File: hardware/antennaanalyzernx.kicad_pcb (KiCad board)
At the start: 2 copper layers, 83.9 x 99 mm, 140 parts, among them J1 Power Connection, J2 SPI Header, J3 Serial Header, J4 GPIO, J5 Conn_Coaxial, J6 TFT Connection, J7 Touch Connection, J8 SD Connection, SW1 Reset, U1 SA612, U10 TLV1117-33, U11 TLV1117-50, U12 ATmega1284P-AU, U2 LM358, U3 Si5351A, U4 SA612, U5 LM358, U6 74HC86, U7 74HC74, U8 LM358, U9 LM324, Y1 27MHz, Y2 16MHz

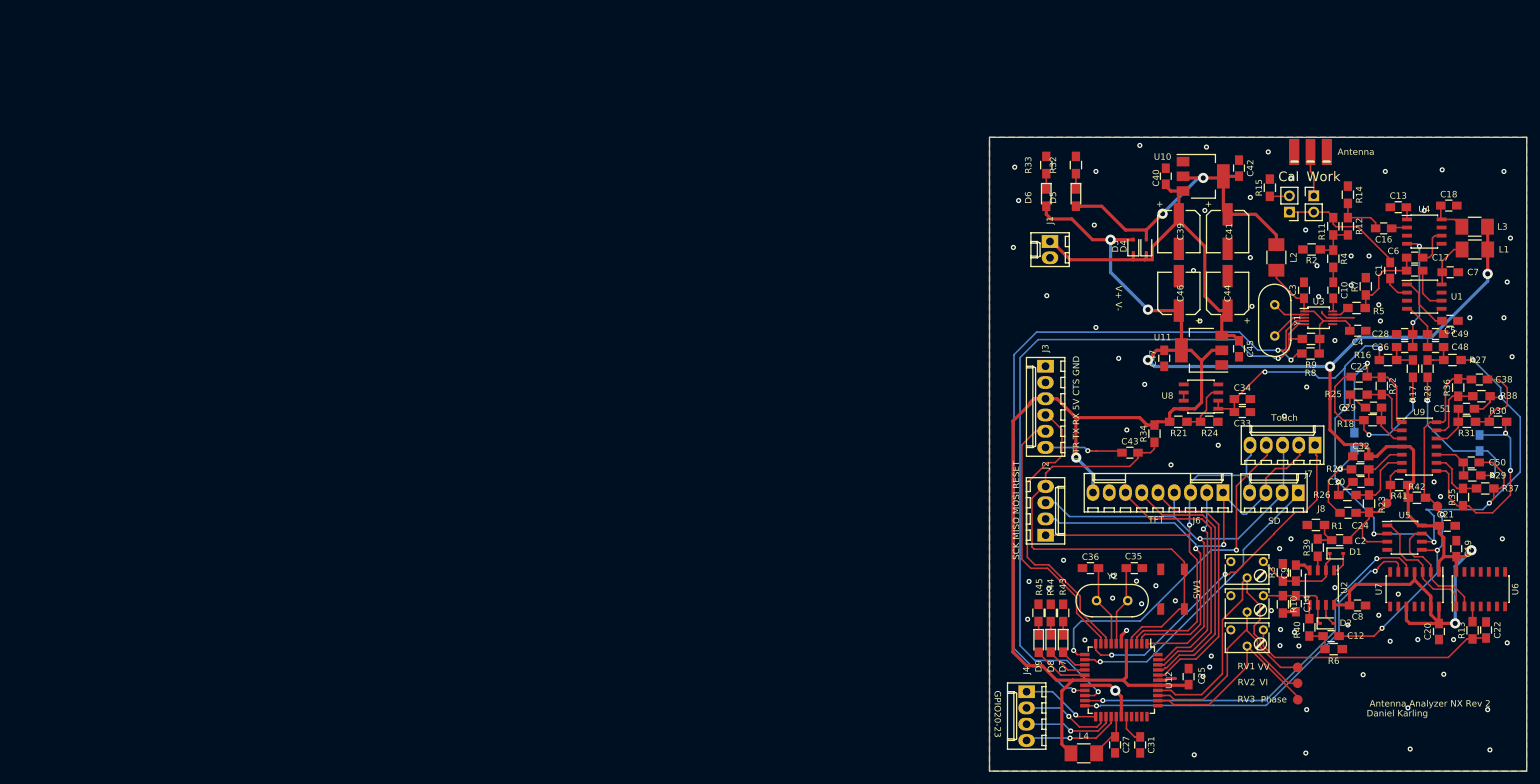
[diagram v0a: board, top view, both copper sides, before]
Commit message: stm32 version
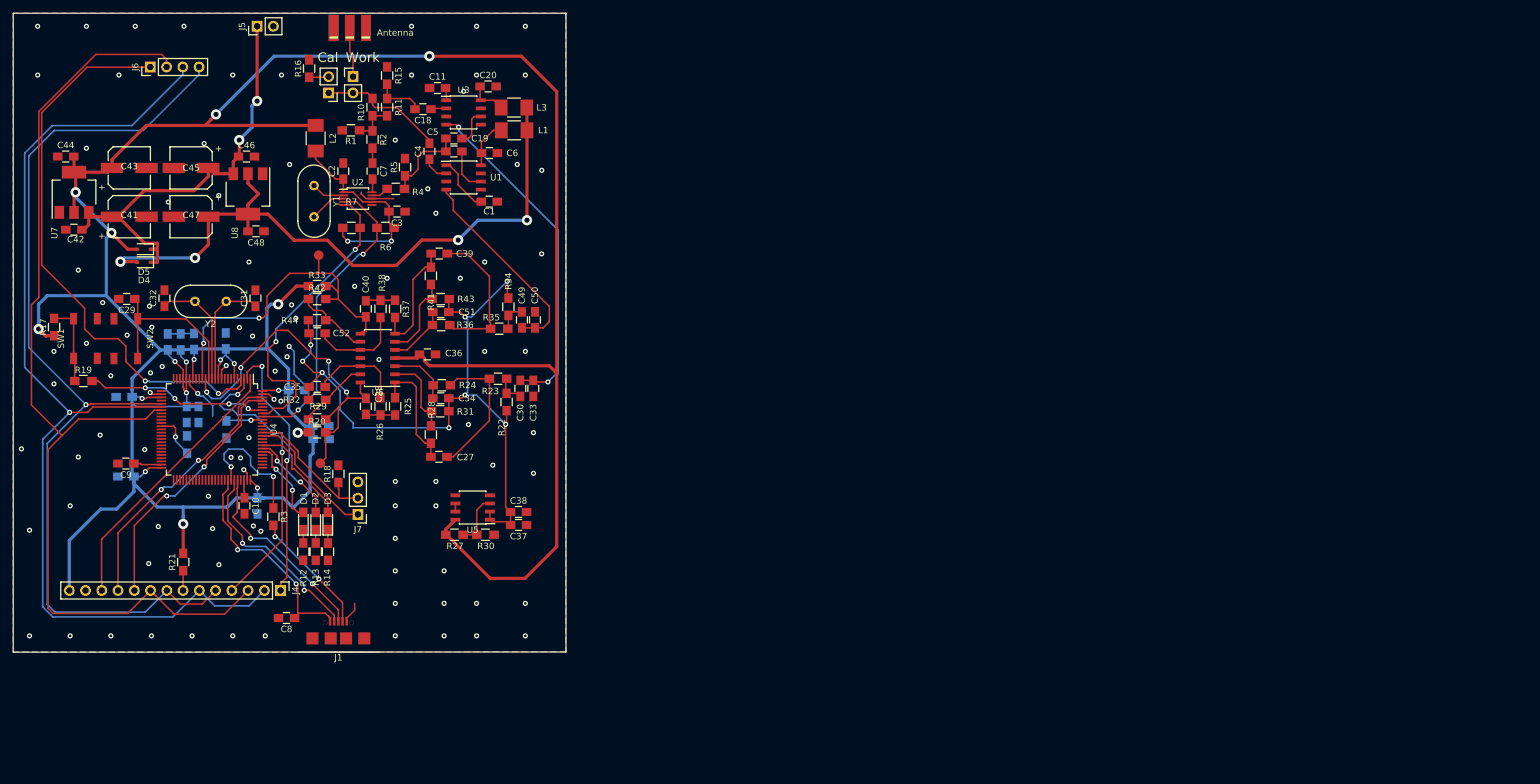
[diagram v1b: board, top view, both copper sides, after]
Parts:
- removed the C19 at (246.8, 103.6)
- removed the C2 at (228.6, 102.3)
- removed the C20 at (244.1, 116.6)
- removed the C27 at (193.5, 134.3)
- removed the C35 at (196.5, 106.7)
- removed the C36 at (189.6, 106.7)
- removed the C43 at (195.8, 88.6)
- removed the D1 at (228.1, 104.4)
- removed the D2 at (226.6, 115.3)
- removed the D5 at (187.4, 48.8)
- removed D6: 5V PWR, LEDs:LED_0805_HandSoldering
- removed the J2 at (182.6, 101.5)
- removed J3: Serial Header, Connectors_Molex:Molex_KK-6410-06_06x2.54mm_Straight
- removed J8: SD Connection, Connectors_Molex:Molex_KK-6410-04_04x2.54mm_Straight
- removed L4: 1u, Inductors_SMD:L_1210_HandSoldering
- removed the R1 at (224.9, 99.9)
- removed the R10 at (219.7, 112.3)
- removed the R13 at (249.3, 116.4)
- removed the R32 at (187.4, 43.7)
- removed the R33 at (182.7, 43.7)
- removed the R34 at (199.6, 85.7)
- removed R39, R40: 10k, Resistors_SMD:R_0805_HandSoldering
- removed the R6 at (227.6, 119.3)
- removed RV1, RV2, RV3: 100k, Potentiometers:Potentiometer_Trimmer_Bourns_3266W
- removed the TP1 at (222.0, 122.2)
- removed the TP2 at (222.0, 124.7)
- removed TP3: TestPoint, Measurement_Points:Measurement_Point_Round-SMD-Pad_Small
- removed U12: ATmega1284P-AU, Housings_QFP:TQFP-44_10x10mm_Pitch0.8mm
- removed the U2 at (225.8, 109.7)
- removed the U7 at (240.3, 110.0)
- removed the U8 at (206.9, 79.9)
- removed U9: LM324, Housings_SOIC:SOIC-14_3.9x8.7mm_Pitch1.27mm
- added C10: 2.2u, Capacitors_SMD:C_0805_HandSoldering, F.Cu at (57.5, 96.9)
- added C13: 100n, Capacitors_SMD:C_0805_HandSoldering, B.Cu at (65.6, 78.9)
- added C15: 100n, Capacitors_SMD:C_0805_HandSoldering, B.Cu at (54.5, 71.2)
- added C16: 100n, Capacitors_SMD:C_0805_HandSoldering, B.Cu at (47.5, 71.3)
- added C17: 100n, Capacitors_SMD:C_0805_HandSoldering, B.Cu at (38.9, 92.4)
- added C23: 4.7u, Capacitors_SMD:C_0805_HandSoldering, B.Cu at (69.4, 86.5)
- added C24: 4.7u, Capacitors_SMD:C_0805_HandSoldering, B.Cu at (69.4, 84.5)
- added C26: 100n, Capacitors_SMD:C_0805_HandSoldering, B.Cu at (38.6, 79.9)
- added C29: 100n, Capacitors_SMD:C_0805_HandSoldering, F.Cu at (39.1, 64.6)
- added C32: 20p, Capacitors_SMD:C_0805_HandSoldering, F.Cu at (45.0, 64.5)
- added J5: Power Connection, Pin_Headers:Pin_Header_Straight_1x02_Pitch2.54mm, F.Cu at (59.4, 22.0)
- added R17: 10k, Resistors_SMD:R_0805_HandSoldering, F.Cu at (27.7, 69.0)
- added R18: 10k, Resistors_SMD:R_0805_HandSoldering, F.Cu at (72.1, 92.0)
- added R19: 10k, Resistors_SMD:R_0805_HandSoldering, F.Cu at (32.3, 77.4)
- added R21: 33, Resistors_SMD:R_0805_HandSoldering, F.Cu at (47.9, 105.7)
- added R8: 10k, Resistors_SMD:R_0805_HandSoldering, B.Cu at (48.5, 87.4)
- added R9: 10k, Resistors_SMD:R_0805_HandSoldering, B.Cu at (54.6, 85.0)
- added SW2: SW_Push, AntennaAnalyzer:Switch, F.Cu at (38.9, 70.8)
- added U4: STM32F407VGTx, Housings_QFP:LQFP-100_14x14mm_Pitch0.5mm, F.Cu at (52.4, 85.0)
- C12: moved to B.Cu
- C14: value 10u -> 100n; moved to B.Cu
- C21, C25: value 100n -> 1u; moved to B.Cu
- C22: value 1u -> 100n; moved to B.Cu
- C31: value 100n -> 20p
- C39: renamed from C37; moved to F.Cu
- C8: value 100n -> 10n
- C9: value 10u -> 2.2u
- J1: value Power Connection -> USB_B_Micro; footprint Connectors_Molex:Molex_KK-6410-02_02x2.54mm_Straight -> AntennaAnalyzer:USB Micro
- J4: value GPIO -> TFT Header; footprint Connectors_Molex:Molex_KK-6410-04_04x2.54mm_Straight -> Pin_Headers:Pin_Header_Straight_1x14_Pitch2.54mm
- J6: value TFT Connection -> SD Header; footprint Connectors_Molex:Molex_KK-6410-09_09x2.54mm_Straight -> Pin_Headers:Pin_Header_Straight_1x04_Pitch2.54mm
- J7: value Touch Connection -> Serial Header; footprint Connectors_Molex:Molex_KK-6410-05_05x2.54mm_Straight -> Pin_Headers:Pin_Header_Straight_1x03_Pitch2.54mm
- R25: renamed from R19; moved to F.Cu
- R3: value 10k -> 0
- SW1: value Reset -> SW_Push; footprint SMA:Switch -> AntennaAnalyzer:Switch
- U5: value LM358 -> MCP602
- U6: value 74HC86 -> MCP604
- Y2: value 16MHz -> Crystal
- moved C21 202.0 mm to (45.5, 71.3), turned to 90 degrees
- moved C22 192.9 mm to (59.5, 97.0), turned to 270 degrees
- moved C9 183.6 mm to (38.9, 90.3), turned to 180 degrees
- moved C44 183.3 mm to (29.5, 42.4), turned to 180 degrees
- moved R44 182.3 mm to (68.8, 68.0), turned to 180 degrees
- moved J6 180.3 mm to (42.7, 28.4), turned to 90 degrees
- moved C12 180.3 mm to (50.3, 82.7), turned to 270 degrees
- moved C52 180.0 mm to (68.8, 70.0), turned to 180 degrees
- moved TP2 179.1 mm to (69.1, 57.8), turned to 270 degrees
- moved R42 178.8 mm to (68.8, 64.6), turned to 180 degrees
- moved C14 177.0 mm to (49.6, 71.3), turned to 90 degrees
- moved U7 176.5 mm to (30.8, 48.0), turned to 90 degrees
- moved U6 176.1 mm to (78.3, 73.9), turned to 180 degrees
- moved R33 175.0 mm to (68.8, 62.6)
- moved C40 174.3 mm to (76.4, 66.2), turned to 90 degrees
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- renumbered C5 to C1, C13 to C11, C16 to C18, C17 to C19, C3 to C2, C18 to C20, C23 to C27, C24 to C28, C4 to C3, C26 to C30, C28 to C33, C29 to C34, C30 to C35, C32 to C36, C33 to C37, C34 to C38, C1 to C4, C38 to C40, C39 to C41, C40 to C42, C41 to C43, C42 to C44, C44 to C45, C45 to C46, C46 to C47, C47 to C48, C48 to C49, C6 to C5, C49 to C50, C50 to C51, C51 to C52, C7 to C6, C10 to C7, D7 to D1, D8 to D2, D9 to D3, D3 to D4, D4 to D5, J5 to J2, R2 to R1, R11 to R10, R12 to R11, R43 to R12, R44 to R13, R45 to R14, R14 to R15, R15 to R16, R4 to R2, R41 to R20, R16 to R22, R17 to R23, R18 to R24, R20 to R26, R21 to R27, R22 to R28, R23 to R29, R24 to R30, R25 to R31, R26 to R32, R42 to R33, R27 to R34, R28 to R35, R29 to R36, R30 to R37, R31 to R38, R5 to R4, R35 to R41, R36 to R42, R37 to R43, R38 to R44, R7 to R5, R8 to R6, R9 to R7, TP4 to TP1, TP5 to TP2, U3 to U2, U4 to U3, U10 to U7, U11 to U8
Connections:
- C1 pad 2: CTS -> GND
- C11 pad 2: CTS -> GND
- C12 pad 1: Net-(C12-Pad1) -> 3.3V
- C12 pad 2: Filtered_VI -> GND
- C14 pad 1: Net-(C14-Pad1) -> 3.3V
- C14 pad 2: CTS -> GND
- C2 pad 2: CTS -> GND
- C20 pad 2: CTS -> GND
- C21 pad 1: CTS -> 3.3V
- C21 pad 2: 5V -> GND
- C22 pad 1: Net-(C22-Pad1) -> 3.3V
- C22 pad 2: CTS -> GND
- C25 pad 1: 5V -> 3.3V
- C25 pad 2: CTS -> GND
- C27 pad 1: Net-(C23-Pad1) -> Net-(C27-Pad1)
- C3 pad 2: CTS -> GND
- C31 pad 1: Net-(C31-Pad1) -> OSC1
- C31 pad 2: CTS -> GND
- C33 pad 2: CTS -> GND
- C34 pad 1: Net-(C29-Pad1) -> Net-(C34-Pad1)
- C34 pad 2: 2.5V -> 1.65V
- C35 pad 1: Net-(C30-Pad1) (its old number) -> Net-(C35-Pad1)
- C35 pad 2: 2.5V -> 1.65V
- C36 pad 1: CTS -> GND
- C36 pad 2: 5V -> 3.3V
- C37 pad 1: 2.5V -> 1.65V
- C37 pad 2: CTS -> GND
- C38 pad 1: 2.5V -> 1.65V
- C38 pad 2: CTS -> GND
- C39 pad 1: Net-(C37-Pad1) -> Net-(C39-Pad1)
- C41 pad 2: CTS -> GND
- C42 pad 2: CTS -> GND
- C43 pad 2: CTS -> GND
- C44 pad 2: CTS -> GND
- C45 pad 2: CTS -> GND
- C46 pad 2: CTS -> GND
- C47 pad 2: CTS -> GND
- C48 pad 2: CTS -> GND
- C50 pad 2: CTS -> GND
- C51 pad 1: Net-(C50-Pad1) -> Net-(C51-Pad1)
- C51 pad 2: 2.5V -> 1.65V
- C52 pad 1: Net-(C51-Pad1) -> Net-(C52-Pad1)
- C52 pad 2: 2.5V -> 1.65V
- C6 pad 2: CTS -> GND
- C8 pad 1: CTS -> VBUS
- C8 pad 2: 5V -> GND
- C9 pad 1: Net-(C9-Pad1) -> VCAP_1
- C9 pad 2: CTS -> GND
- J1 pad 1: VIN -> VBUS
- J1 pad 2: CTS -> USB_DM
- J2 pad 2: CTS -> GND
- J4 pad 1: GPIO20 -> TOUCH_IRQ
- J4 pad 2: GPIO21 -> MISO
- J4 pad 3: GPIO22 -> MOSI
- J4 pad 4: GPIO23 -> TOUCH_CS
- J6 pad 1: MISO -> SD_CS
- J6 pad 2: TFT_LED -> MOSI
- J6 pad 3: SCK -> MISO
- J6 pad 4: MOSI -> SCK
- J7 pad 1: TOUCH_IRQ -> TX
- J7 pad 2: MISO -> RX
- J7 pad 3: MOSI -> GND
- R1 pad 2: CTS -> GND
- R12 pad 2: CTS -> GND
- R13 pad 2: CTS -> GND
- R14 pad 2: CTS -> GND
- R15 pad 2: CTS -> GND
- R16 pad 2: CTS -> GND
- R20 pad 1: 5V -> 3.3V
- R22 pad 1: 2.5V -> 1.65V
- R24 pad 1: Net-(C29-Pad1) -> Net-(C34-Pad1)
- R25 pad 2: Net-(C23-Pad1) -> Net-(C27-Pad1)
- R26 pad 1: Net-(C30-Pad1) (its old number) -> Net-(C35-Pad1)
- R27 pad 1: 5V -> 3.3V
- R27 pad 2: Net-(R21-Pad2) -> Net-(R27-Pad2)
- R28 pad 1: Net-(C23-Pad1) -> Net-(C27-Pad1)
- R28 pad 2: Net-(R22-Pad2) -> Net-(R28-Pad2)
- R29 pad 2: Net-(R23-Pad2) -> Net-(R29-Pad2)
- R3 pad 1: Net-(C9-Pad1) -> USB_ID
- R3 pad 2: CTS -> Net-(J1-Pad4)
- R30 pad 1: Net-(R21-Pad2) -> Net-(R27-Pad2)
- R30 pad 2: CTS -> GND
- R31 pad 1: Net-(R22-Pad2) -> Net-(R28-Pad2)
- R31 pad 2: 2.5V -> 1.65V
- R32 pad 1: Net-(R23-Pad2) -> Net-(R29-Pad2)
- R32 pad 2: 2.5V -> 1.65V
- R33 pad 1: 5V -> 3.3V
- R34 pad 1: 2.5V -> 1.65V
- R36 pad 1: Net-(C50-Pad1) -> Net-(C51-Pad1)
- R37 pad 2: Net-(C37-Pad1) -> Net-(C39-Pad1)
- R38 pad 1: Net-(C51-Pad1) -> Net-(C52-Pad1)
- R41 pad 1: Net-(C37-Pad1) -> Net-(C39-Pad1)
- R41 pad 2: Net-(R35-Pad2) -> Net-(R41-Pad2)
- R42 pad 2: Net-(R36-Pad2) -> Net-(R42-Pad2)
- R43 pad 1: Net-(R35-Pad2) -> Net-(R41-Pad2)
- R43 pad 2: 2.5V -> 1.65V
- R44 pad 1: Net-(R36-Pad2) -> Net-(R42-Pad2)
- R44 pad 2: 2.5V -> 1.65V
- R5 pad 2: CTS -> GND
- SW1 pad 1: RESET -> Net-(R17-Pad2)
- SW1 pad 2: CTS -> GND
- U1 pad 3: CTS -> GND
- U2 pad 8: CTS -> GND
- U3 pad 3: CTS -> GND
- U5 pad 1: Net-(U5-Pad1) -> 1.65V
- U5 pad 2: 2.5V -> 1.65V
- U5 pad 3: Filtered_VV -> Net-(R27-Pad2)
- U5 pad 4: CTS -> GND
- U5 pad 5: Filtered_VI -> GND
- U5 pad 6: 2.5V -> Net-(U5-Pad6)
- U5 pad 7: Net-(U5-Pad7) -> Net-(U5-Pad6)
- U5 pad 8: 5V -> 3.3V
- U6 pad 1: Net-(U5-Pad1) -> Net-(C27-Pad1)
- U6 pad 10: CTS -> Net-(C52-Pad1)
- U6 pad 11: (no net) -> GND
- U6 pad 12: CTS -> Net-(C35-Pad1)
- U6 pad 13: CTS -> Net-(R29-Pad2)
- U6 pad 14: 5V -> Filtered_VV
- U6 pad 2: Net-(U5-Pad7) -> Net-(R28-Pad2)
- U6 pad 3: Net-(R13-Pad2) -> Net-(C34-Pad1)
- U6 pad 4: CTS -> 3.3V
- U6 pad 5: CTS -> Net-(C51-Pad1)
- U6 pad 6: (no net) -> Net-(R41-Pad2)
- U6 pad 7: CTS -> Net-(C39-Pad1)
- U6 pad 8: (no net) -> Filtered_VI
- U6 pad 9: CTS -> Net-(R42-Pad2)
- U7 pad 1: CTS -> GND
- U8 pad 1: CTS -> GND
- Y2 pad 1: Net-(C35-Pad2) -> OSC1
- Y2 pad 2: Net-(C36-Pad2) -> OSC2
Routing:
- net 3.3V: track 52.6 -> 498.1 mm, vias 2 -> 18
- net 5V: track 368.8 -> 106.1 mm, vias 8 -> 4
- net 2.5V: track 150.8 -> 0.00 mm, vias 9 -> 0
- net 1.65V: track 0.00 -> 109.5 mm, vias 0 -> 8
- net MOSI: track 77.7 -> 159.5 mm, vias 1 -> 0
- net SCK: track 73.4 -> 151.3 mm
- net MISO: track 83.4 -> 160.1 mm, vias 2 -> 1
- net RESET: track 75.9 -> 0.00 mm
- net SCL: track 116.1 -> 47.3 mm, vias 3 -> 2
- net SDA: track 115.1 -> 47.6 mm
- net Capacitive_Sign: track 63.8 -> 0.00 mm, vias 2 -> 0
- net Inductive_Sign: track 62.6 -> 0.00 mm, vias 2 -> 0
- net VV_Peak: track 47.9 -> 0.00 mm
- net SD_CS: track 46.0 -> 88.0 mm, vias 1 -> 2
- net Net-(C22-Pad1): track 39.3 -> 0.00 mm
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- added copper zone on B.Cu, net GND
- added copper zone on F.Cu, net GND
- removed copper zone on B.Cu, net CTS
- removed copper zone on F.Cu, net CTS
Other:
- board size 83.9 x 99 mm -> 86.4 x 99.8 mm
- board text removed: "Antenna Analyzer NX Rev 2"
- board text removed: "DTR TX RX 5V CTS GND"
- board text removed: "Daniel Karling"
- board text removed: "GPIO20-23"
- board text removed: "Phase"
- board text removed: "SCK MISO MOSI RESET"
- board text removed: "SD"
- board text removed: "TFT"
- board text removed: "Touch"
- board text removed: "V+ V-"
- board text removed: "VI"
- board text removed: "VV"
